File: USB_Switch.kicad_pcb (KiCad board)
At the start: 2 copper layers, 42 x 61 mm, 30 parts, among them J1 Conn_01x06, J2 USB_IN, J3 USB_OUT, J4 Conn_01x08, J5 USB_OUT, Q1 Q_NMOS_GDS, Q2 Q_NMOS_GDS, SW1 PRGM, U1 AMS1117-3.3, U2 INA219AxD, U3 INA219AxD, U4 ESP-12F

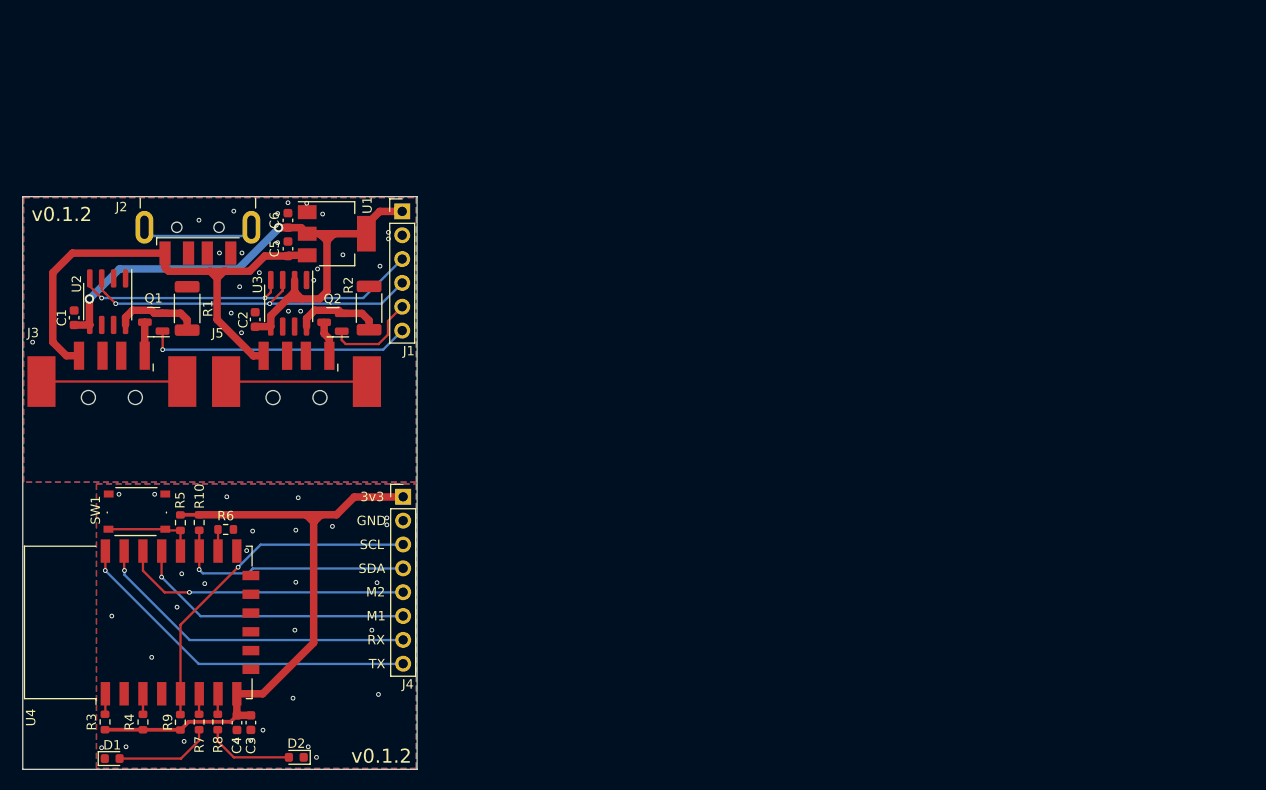
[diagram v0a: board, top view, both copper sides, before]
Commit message: Updated to v0.2.0
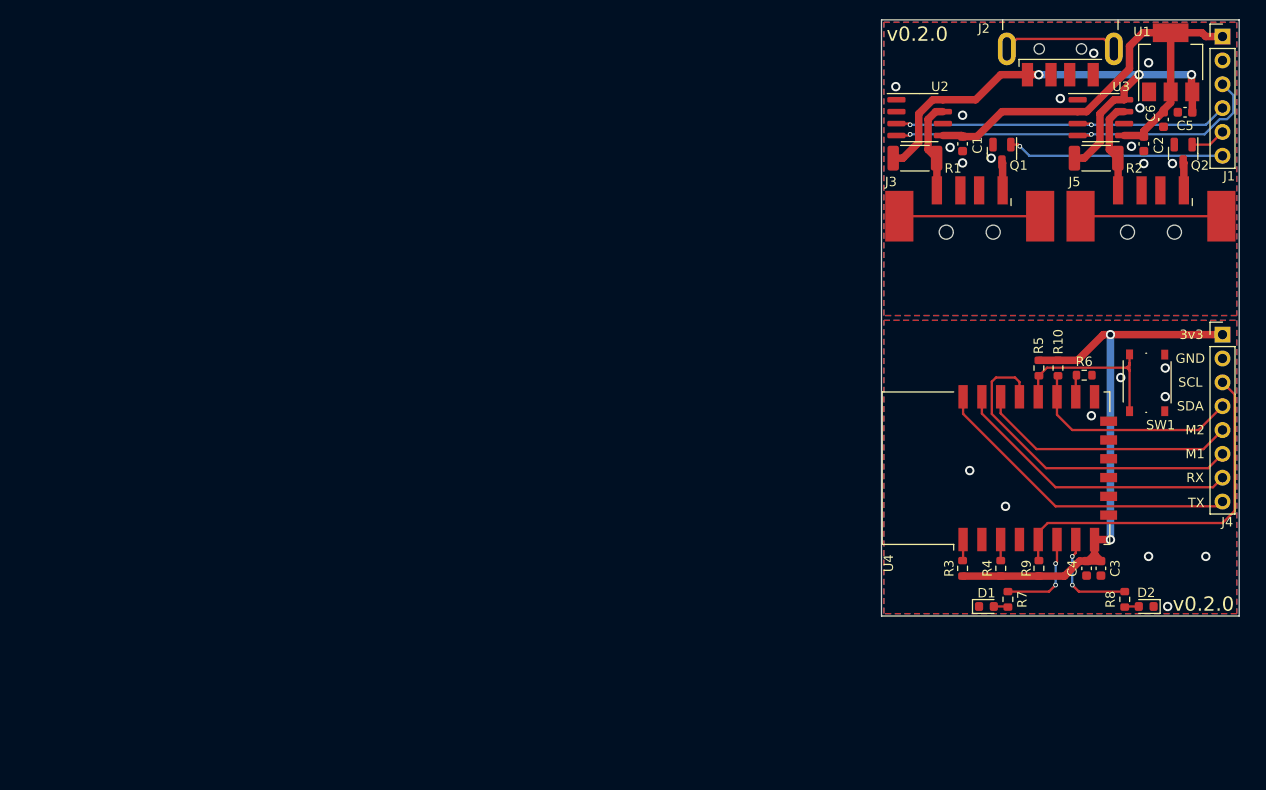
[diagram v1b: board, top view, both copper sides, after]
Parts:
- moved SW1 108.4 mm to (155.2, 102.1), turned to 90 degrees
- moved R8 97.5 mm to (152.9, 125.2)
- moved C5 96.7 mm to (159.3, 73.3), turned to 180 degrees
- moved C2 96.5 mm to (154.9, 76.7), turned to -90 degrees
- moved C1 96.4 mm to (135.6, 76.7), turned to -90 degrees
- moved D1 94.5 mm to (138.2, 126.0)
- moved C6 93.9 mm to (157.0, 74.1), turned to -90 degrees
- moved J2 93.8 mm to (146.1, 59.7)
- moved J3 93.1 mm to (136.4, 83.3)
- moved R10 92.9 mm to (145.8, 100.6)
- moved R5 92.9 mm to (143.8, 100.6)
- moved R6 92.9 mm to (148.6, 101.3)
- moved R9 92.9 mm to (143.8, 121.9)
- moved U4 92.8 mm to (139.2, 111.3)
- moved R4 92.8 mm to (139.7, 121.9)
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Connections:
- net /MOSFET Board/SW_GND_1 renamed /MOSFET Board/Switch Circuit/PRE_MOS
- net /MOSFET Board/SW_GND_2 renamed /MOSFET Board/Switch Circuit1/PRE_MOS
- J3 pad 1: /MOSFET Board/5V_IN -> /MOSFET Board/Switch Circuit/POST_RES
- J5 pad 1: /MOSFET Board/5V_IN -> /MOSFET Board/Switch Circuit1/POST_RES
- Q1 pad 3: /MOSFET Board/5V_PRER_1 -> GND
- Q2 pad 3: /MOSFET Board/5V_PRER_2 -> GND
- R1 pad 1: /MOSFET Board/5V_PRER_1 -> /MOSFET Board/5V_IN
- R1 pad 2: GND -> /MOSFET Board/Switch Circuit/POST_RES
- R2 pad 1: /MOSFET Board/5V_PRER_2 -> /MOSFET Board/5V_IN
- R2 pad 2: GND -> /MOSFET Board/Switch Circuit1/POST_RES
- U2 pad 7: GND -> /MOSFET Board/Switch Circuit/POST_RES
- U2 pad 8: /MOSFET Board/5V_PRER_1 -> /MOSFET Board/5V_IN
- U3 pad 7: GND -> /MOSFET Board/Switch Circuit1/POST_RES
- U3 pad 8: /MOSFET Board/5V_PRER_2 -> /MOSFET Board/5V_IN
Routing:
- net /MOSFET Board/M_3v3: track 63.6 -> 50.4 mm, vias 2 -> 0
- net /MOSFET Board/Switch Circuit1/POST_RES: track 0.00 -> 9.87 mm
- net /MOSFET Board/Switch Circuit/POST_RES: track 0.00 -> 9.87 mm
- net /MOSFET Board/5V_PRER_2: track 9.33 -> 0.00 mm
- net /MOSFET Board/5V_PRER_1: track 9.21 -> 0.00 mm
- net Net-(R5-Pad1): track 9.92 -> 19.0 mm
- net Net-(D1-Pad2): track 10.3 -> 1.52 mm
- net /Control Board/LED_2: track 2.20 -> 10.9 mm, vias 0 -> 2
- net /Control Board/LED_1: track 2.19 -> 10.3 mm, vias 0 -> 2
- net Net-(D2-Pad2): track 9.36 -> 1.52 mm
- net /MOSFET Board/M2_TOGGLE: track 10.1 -> 3.80 mm
- net /Control Board/M1_TOGGLE: track 30.2 -> 35.9 mm, vias 1 -> 0
- net /MOSFET Board/M1_TOGGLE: track 28.3 -> 23.0 mm
- net /Control Board/C_3v3: track 68.6 -> 63.3 mm, vias 0 -> 2
- net /Control Board/C_TX: track 37.9 -> 33.7 mm, vias 1 -> 0
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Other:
- board size 42 x 61 mm -> 38.1 x 63.5 mm
- board text added: "v0.2.0"
- board text removed: "v0.1.2"
